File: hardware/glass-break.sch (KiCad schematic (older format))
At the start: 31 parts, among them P1 USB_OTG, SW1 SW_PUSH, SW2 SW_PUSH, U1 esp12, U11 SPX3819, U2 OP275, U3 admp401

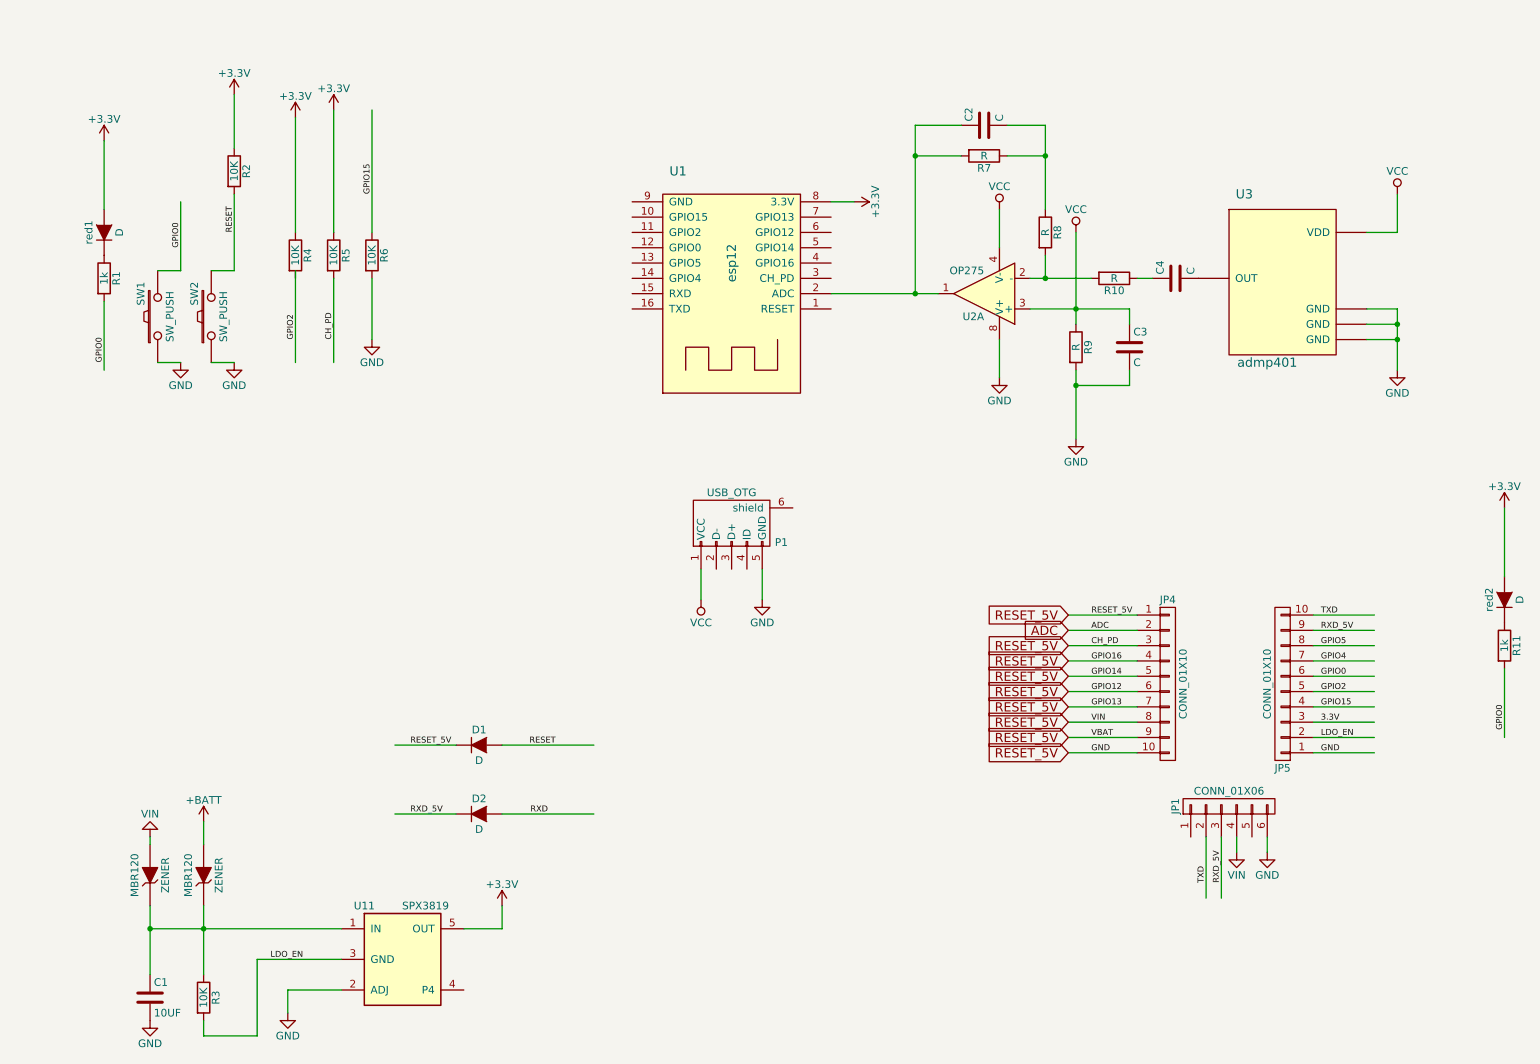
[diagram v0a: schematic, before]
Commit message: update
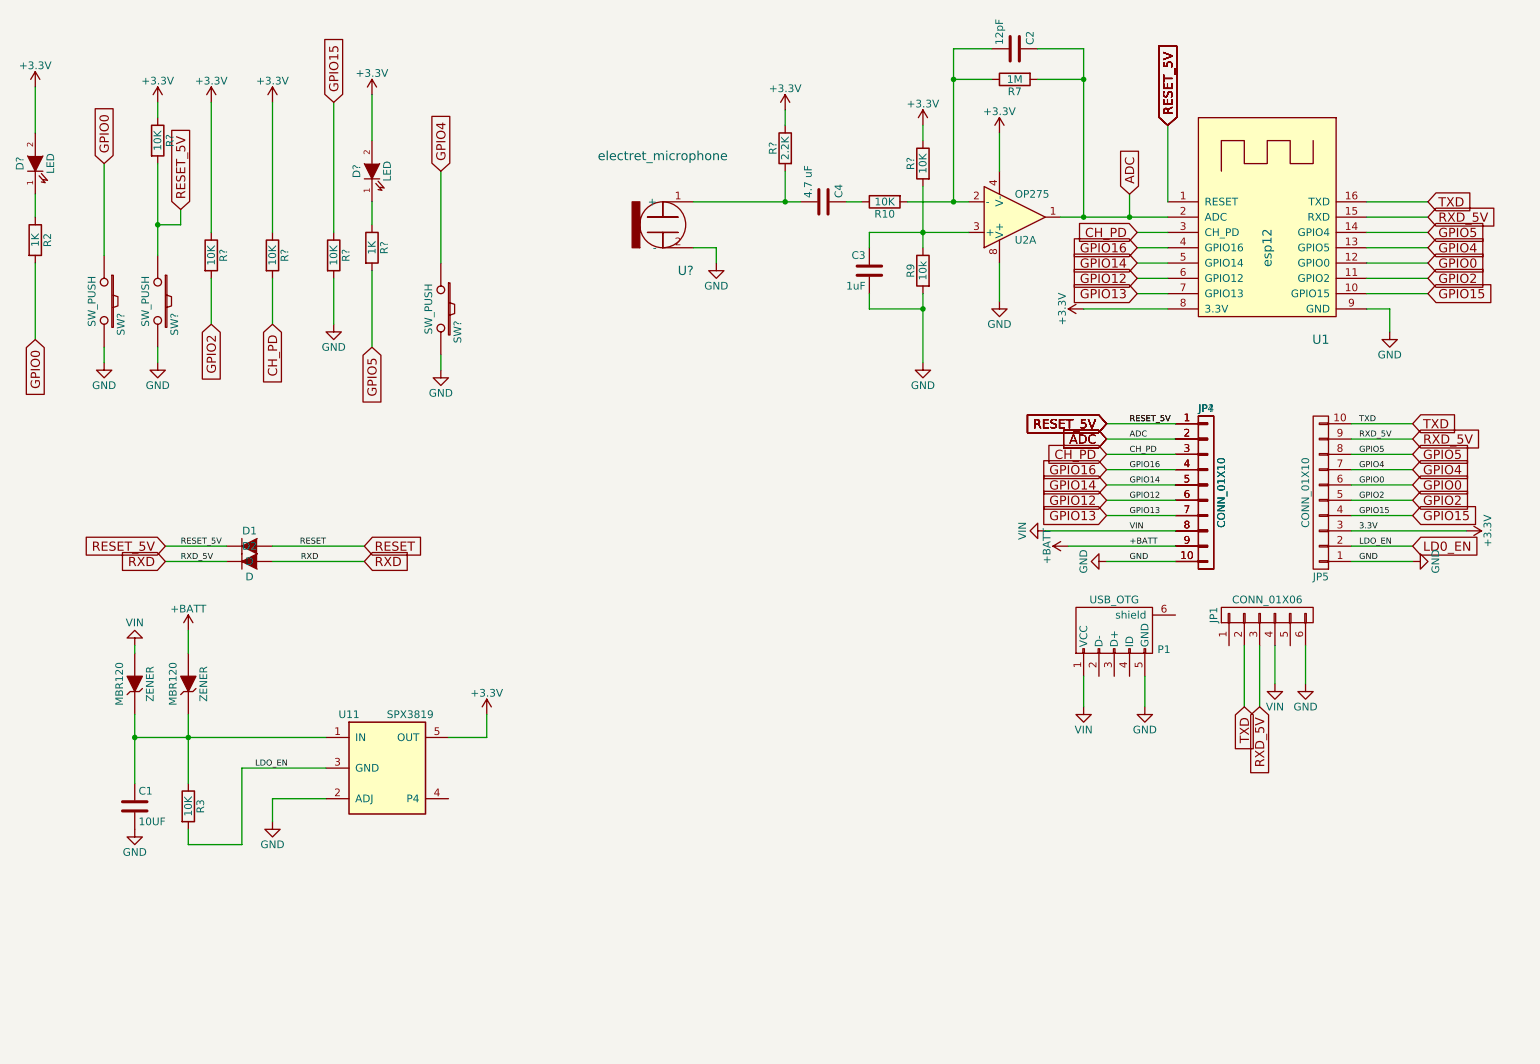
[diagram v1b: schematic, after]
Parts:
- removed R1, R11: 1k, symbol R
- removed R4, R5, R6: 10K, symbol R
- removed R8: R, symbol R
- removed SW1, SW2: SW_PUSH, symbol SW_PUSH
- removed U3: admp401, symbol admp401
- removed red1, red2: D, symbol D
- added D? (x2): LED, symbol LED
- added JP?: CONN_01X10, symbol CONN_01X10
- added R? (x5): 10K, symbol R
- added R?: 1K, symbol R
- added R?: 2.2K, symbol R
- added SW? (x3): SW_PUSH, symbol SW_PUSH
- added U?: electret_microphone, symbol electret_microphone
- C2: value C -> 12pF
- C3: value C -> 1uF
- C4: value C -> 4.7 uF
- R10: value R -> 10K
- R2: value 10K -> 1K
- R7: value R -> 1M
- R9: value R -> 10k
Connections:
- net labels added: LD0_EN
- net labels removed: VBAT, VCC
- wire segments 85 -> 104
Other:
- moved on the sheet: C1, C2, C3, C4, D1, D2, JP1, JP4, JP5, MBR120, P1, R10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
